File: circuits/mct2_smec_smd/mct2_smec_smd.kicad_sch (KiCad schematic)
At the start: 8 parts

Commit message: 20250306-1
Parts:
- added J?: Conn_02x15_Odd_Even, symbol Connector_Generic:Conn_02x15_Odd_Even
- U? (x7): value ~ -> GW1N-UV2QN48C7/I6; footprint (none) -> Package_DFN_QFN:QFN-48-1EP_6x6mm_P0.4mm_EP4.2x4.2mm_ThermalVias
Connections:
- net GND: now also J?.1 (Pin_1), J?.10 (Pin_10), J?.13 (Pin_13), J?.16 (Pin_16), J?.19 (Pin_19), J?.2 (Pin_2), J?.20 (Pin_20), J?.25 (Pin_25), J?.30 (Pin_30), J?.6 (Pin_6), J?.7 (Pin_7); no longer J?.29 (Pin_29), J?.3 (Pin_3), J?.36 (Pin_36)
- net VDD: no longer J?.4 (Pin_4)
- net DISP_B0: no longer names the net of J?.21 (Pin_21)
- net DISP_B0: no longer U?.28 (IOB5B/SO)
- net DISP_B1: no longer names the net of J?.22 (Pin_22)
- net DISP_B1: no longer U?.29 (IOB5A/SCLK)
- net DISP_B2: no longer names the net of J?.23 (Pin_23)
- net DISP_B2: no longer U?.30 (IOB7B/GCLKC_4)
- net DISP_B3: no longer names the net of J?.24 (Pin_24)
- net DISP_B3: no longer U?.31 (IOB7A/GCLKT_4)
- net DISP_B4: no longer names the net of J?.25 (Pin_25)
- net DISP_B4: no longer U?.32 (IOB13B)
- net DISP_B5: no longer names the net of J?.26 (Pin_26)
- net DISP_B5: no longer U?.33 (IOB13A)
- net DISP_B6: no longer names the net of J?.27 (Pin_27)
- net DISP_B6: no longer U?.34 (IOB18A/SSPI_CS_N)
- net DISP_B7: no longer names the net of J?.28 (Pin_28)
- net DISP_B7: no longer U?.35 (IOB18B/SI)
- net DISP_DE: no longer names the net of J?.34 (Pin_34)
- net DISP_DE: no longer U?.27 (IOL17A)
- net DISP_DISP: no longer names the net of J?.31 (Pin_31)
- net DISP_G0: no longer names the net of U?.44 (IOR3B/D3)
- net DISP_G0: no longer J?.13 (Pin_13)
- net DISP_G1: no longer names the net of U?.45 (IOR3A/D2)
- net DISP_G1: no longer J?.14 (Pin_14)
- net DISP_G2: no longer names the net of U?.46 (IOR1B)
- net DISP_G2: no longer J?.15 (Pin_15)
- net DISP_G3: no longer names the net of U?.47 (IOR1A)
- net DISP_G3: no longer J?.16 (Pin_16)
- net DISP_G4: no longer names the net of U?.38 (IOR13A)
- net DISP_G4: no longer J?.17 (Pin_17)
- net DISP_G5: no longer names the net of U?.39 (IOR13B)
- net DISP_G5: no longer J?.18 (Pin_18)
- net DISP_G6: no longer names the net of U?.40 (IOR11B/GCLKC_2)
- net DISP_G6: no longer J?.19 (Pin_19)
- net DISP_G7: no longer names the net of U?.41 (IOR11A/GCLKT_2)
- net DISP_G7: no longer J?.20 (Pin_20)
- net DISP_HSYNC: no longer names the net of J?.32 (Pin_32)
- net DISP_HSYNC: no longer U?.23 (IOL15A)
- net DISP_PCLK: no longer names the net of J?.30 (Pin_30)
- net DISP_PCLK: no longer U?.22 (IOL15B)
- net DISP_R0: no longer names the net of U?.6 (IOT11A/GCLKT_0)
- net DISP_R0: no longer J?.5 (Pin_5)
- net DISP_R1: no longer names the net of U?.7 (IOT11B/GCLKC_0)
- net DISP_R1: no longer J?.6 (Pin_6)
- net DISP_R2: no longer names the net of U?.8 (IOT9B/TMS)
- net DISP_R2: no longer J?.7 (Pin_7)
- net DISP_R3: no longer names the net of U?.9 (IOT9A/TCK)
- net DISP_R3: no longer J?.8 (Pin_8)
- net DISP_R4: no longer names the net of U?.10 (IOT7B/TDI)
- net DISP_R4: no longer J?.9 (Pin_9)
- net DISP_R5: no longer names the net of U?.11 (IOT7A/TDO)
- net DISP_R5: no longer J?.10 (Pin_10)
- net DISP_R6: no longer names the net of U?.13 (IOT2A/MODE0)
- net DISP_R6: no longer J?.11 (Pin_11)
- net DISP_R7: no longer names the net of U?.48 (IOT16B/RECONFIG_N)
- net DISP_R7: no longer J?.12 (Pin_12)
- net DISP_VSYNC: no longer names the net of J?.33 (Pin_33)
- net DISP_VSYNC: no longer U?.24 (IOL17B)
- new net DISP_ID: J?.14 (Pin_14)
- new net DISP_IO: J?.8 (Pin_8)
- new net DISP_MTP_VPP: J?.23 (Pin_23)
- new net DISP_RST: J?.12 (Pin_12)
- new net DISP_VBAT: J?.27 (Pin_27), J?.29 (Pin_29)
- new net DISP_VCI_EN: J?.4 (Pin_4)
- new net MIPI_CLK_N: J?.3 (Pin_3), U?.22 (IOL15B)
- new net MIPI_CLK_P: J?.5 (Pin_5), U?.23 (IOL15A)
- new net MIPI_D0_N: J?.15 (Pin_15), U?.24 (IOL17B)
- new net MIPI_D0_P: J?.17 (Pin_17), U?.27 (IOL17A)
- new net MIPI_TE: J?.21 (Pin_21)
- new net TP_INT: J?.24 (Pin_24)
- new net TP_RST: J?.22 (Pin_22)
- new net TP_SCL: J?.28 (Pin_28)
- new net TP_SDA: J?.26 (Pin_26)
- new net TP_VCC: J?.18 (Pin_18)
- no-connect marks 5 -> 2
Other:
- note added: "1"
- note added: "2025-02-24 - 2025-03-02"
- note added: "40"
- note added: "BANK0"
- note added: "BANK1"
- note added: "BANK2"
- note added: "BANK3"
- note added: "BANK4"
- note added: "BANK5"
- note added: "Datasheet for TOH323XVT-01C has the pinout inconsistent for: Pin 22 - Drawing: CTP_RST - Module Interface: GND"
- note added: "IOL15A/B and IOL17A/B should support MIPI per LVDS support in UG171 and DS100"
- note added: "Make sure to also refer to the Raydium RM690C0 datasheet for pin definitions"
- note added: "Raydium RM690C0 Datasheet Rev. V0.1 states a maximum DSI bandwidth of 550Mbps per lane. GOWIN DS100 states a maximum MIPI DSI TX rate of 2Gbps per lane. Width x Length x Bit depth x FPS = 262 x 928 x 24 x 60 = 350115840 = 333.90 Mibps/350.12 Mbps"
- note added: "TODO: - Should VPP/MTP be exposed via a separate header for in-circuit programming?"
- note removed: "2025-02-24 - 2025-02-24"
- moved on the sheet: J?, U?A, U?B, U?C, U?D, U?E, U?F, U?G

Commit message: 20250306-2
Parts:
- added J2: Conn_01x07, Connector_PinHeader_2.54mm:PinHeader_1x07_P2.54mm_Vertical, symbol Connector_Generic:Conn_01x07
- added NT1, NT2, NT3, NT4: NetTie_2, symbol Device:NetTie_2
- J1: renamed from J?; value Conn_01x40_Socket -> Input 1x40 FPC; footprint (none) -> Connector_FFC-FPC:TE_4-1734839-0_1x40-1MP_P0.5mm_Horizontal
- J3: renamed from J?; footprint (none) -> Connector_PinHeader_2.54mm:PinHeader_2x10_P2.54mm_Vertical_SMD
- gave numbers to parts that had none: 1
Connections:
- net GND: now also J1.29 (Pin_29), J1.3 (Pin_3), J1.36 (Pin_36), U1.2 (VSS), U1.26 (VSS)
- net JTAG_JTAGSEL_N: now also J2.1 (Pin_1), NT1.2
- net JTAG_MODE0: now also U1.13 (IOT2A/MODE0), J2.6 (Pin_6)
- net JTAG_RECONFIG_N: now also U1.48 (IOT16B/RECONFIG_N), J2.7 (Pin_7)
- net JTAG_TCK: now also J2.3 (Pin_3), NT3.2
- net JTAG_TDI: now also J2.4 (Pin_4), NT4.2
- net JTAG_TDO: now also U1.11 (IOT7A/TDO), J2.5 (Pin_5)
- net JTAG_TMS: now also J2.2 (Pin_2), NT2.2
- net MIPI_TE: now also U1.21 (IOL11B)
- net RGB_B0: now also J1.21 (Pin_21), U1.28 (IOB5B/SO)
- net RGB_B1: now also J1.22 (Pin_22), U1.29 (IOB5A/SCLK)
- net RGB_B2: now also J1.23 (Pin_23), U1.30 (IOB7B/GCLKC_4)
- net RGB_B3: now also J1.24 (Pin_24), U1.31 (IOB7A/GCLKT_4)
- net RGB_B4: now also J1.25 (Pin_25), U1.32 (IOB13B)
- net RGB_B5: now also J1.26 (Pin_26), U1.33 (IOB13A)
- net RGB_B6: now also J1.27 (Pin_27), U1.34 (IOB18A/SSPI_CS_N)
- net RGB_B7: now also J1.28 (Pin_28), U1.35 (IOB18B/SI)
- net RGB_DE: now also J1.34 (Pin_34), U1.17 (IOL5B/LPLL_C_in)
- net RGB_G0: now also J1.13 (Pin_13), U1.3 (IOT16A/JTAGSEL_N), NT1.1
- net RGB_G1: now also J1.14 (Pin_14), U1.4 (IOT14B/GCLKC_1/SDA)
- net RGB_G2: now also J1.15 (Pin_15), U1.5 (IOT14A/GCLKT_1/SCL)
- net RGB_G3: now also J1.16 (Pin_16), U1.6 (IOT11A/GCLKT_0)
- net RGB_G4: now also J1.17 (Pin_17), U1.7 (IOT11B/GCLKC_0)
- net RGB_G5: now also J1.18 (Pin_18), U1.8 (IOT9B/TMS), NT2.1
- net RGB_G6: now also J1.19 (Pin_19), U1.9 (IOT9A/TCK), NT3.1
- net RGB_G7: now also J1.20 (Pin_20), U1.10 (IOT7B/TDI), NT4.1
- net RGB_HSYNC: now also J1.32 (Pin_32), U1.15 (IOL4A/LPLL_T_fb)
- net RGB_PCLK: now also J1.30 (Pin_30), U1.14 (IOL4B/LPLL_C_fb)
- net RGB_R0: now also J1.5 (Pin_5), U1.38 (IOR13A)
- net RGB_R1: now also J1.6 (Pin_6), U1.39 (IOR13B)
- net RGB_R2: now also J1.7 (Pin_7), U1.40 (IOR11B/GCLKC_2)
- net RGB_R3: now also J1.8 (Pin_8), U1.41 (IOR11A/GCLKT_2)
- net RGB_R4: now also J1.9 (Pin_9), U1.42 (IOR5B/MO/D6)
- net RGB_R5: now also J1.10 (Pin_10), U1.43 (IOR5A/MI/D7)
- net RGB_R6: now also J1.11 (Pin_11), U1.44 (IOR3B/D3)
- net RGB_R7: now also J1.12 (Pin_12), U1.45 (IOR3A/D2)
- net RGB_VSYNC: now also J1.33 (Pin_33), U1.16 (IOL5A/LPLL_T_in)
- net VDD: now also J1.4 (Pin_4)
- net RGB_EN: now reaches U1.18 (IOL6A/GCLKT_7)
- net RGB_EN: now also J1.31 (Pin_31)
- net DISP_IO renamed DISP_IOVCC
- net DISP_MTP_VPP: no longer names the net of J3.23 (Pin_23)
- no-connect marks 2 -> 8
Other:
- note added: "2025-02-24 - 2025-03-06"
- note added: "TODO: replace pin header with proper footprint for OK-23GF030-04"
- note removed: "2025-02-24 - 2025-03-02"
- note removed: "Datasheet for TOH323XVT-01C has the pinout inconsistent for: Pin 22 - Drawing: CTP_RST - Module Interface: GND"
- note removed: "TODO: - Should VPP/MTP be exposed via a separate header for in-circuit programming?"
- note removed: "TODO: find out if these pins have important alternate functions and move data pins if they do"
- moved on the sheet: J1, U1A, U1C, U1D, U1E, U1F, U1G

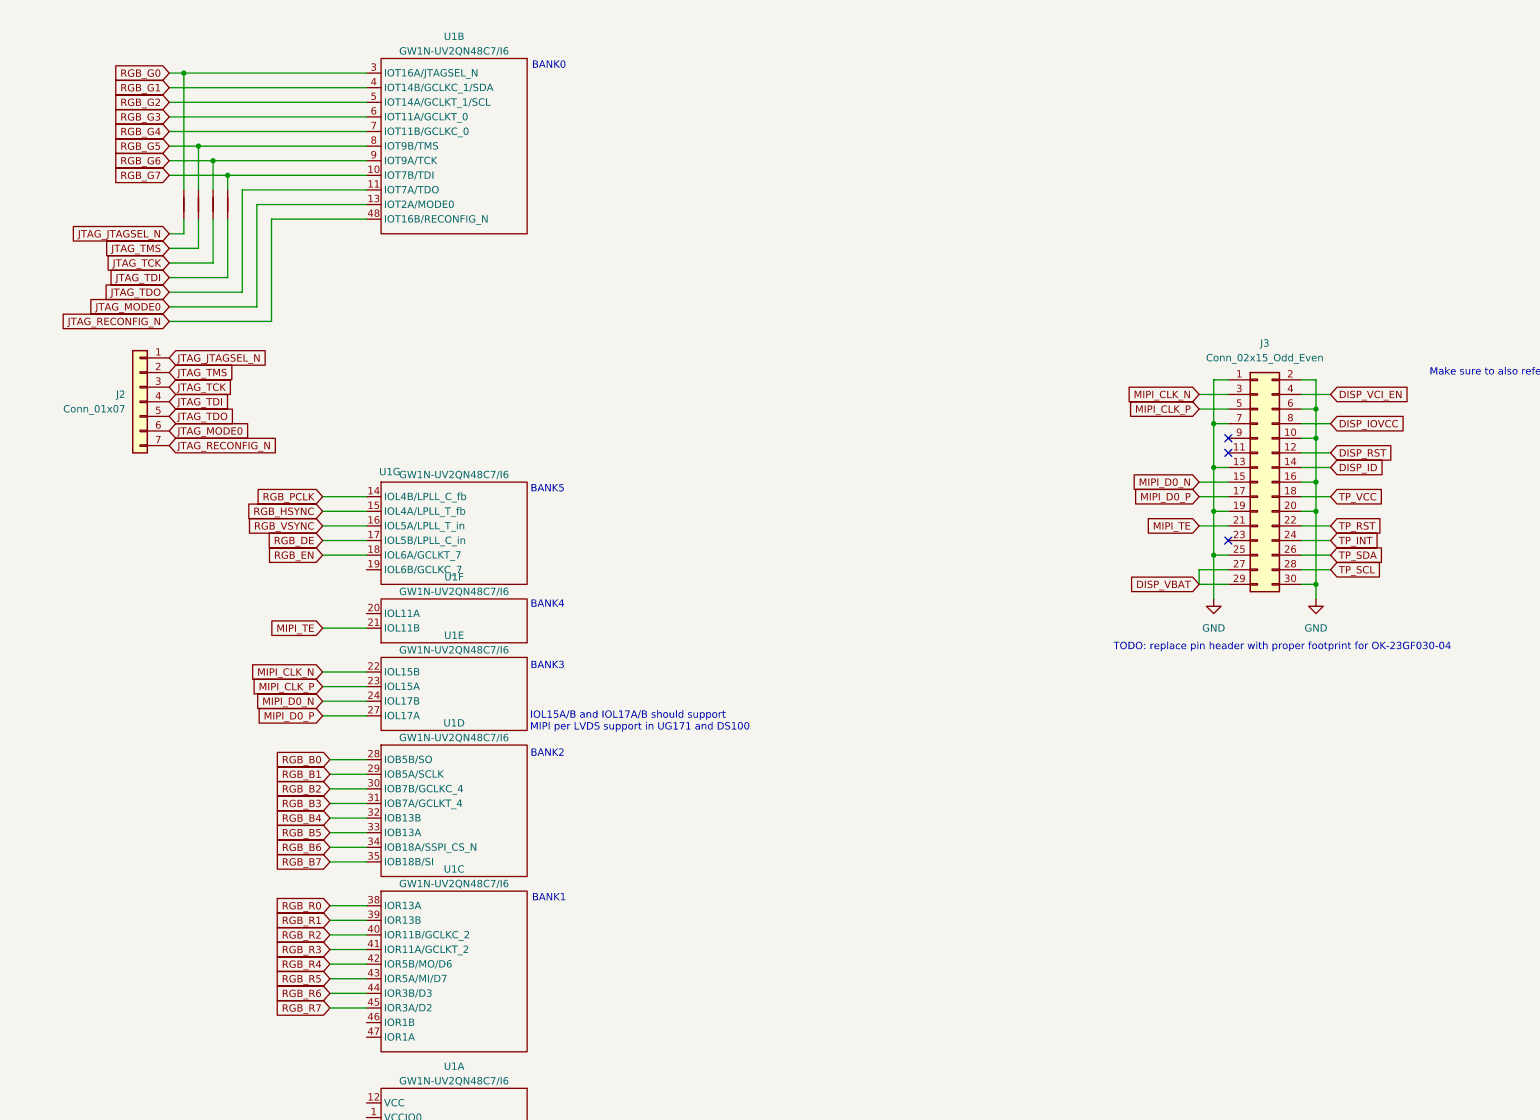
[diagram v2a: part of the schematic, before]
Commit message: 20250311-1
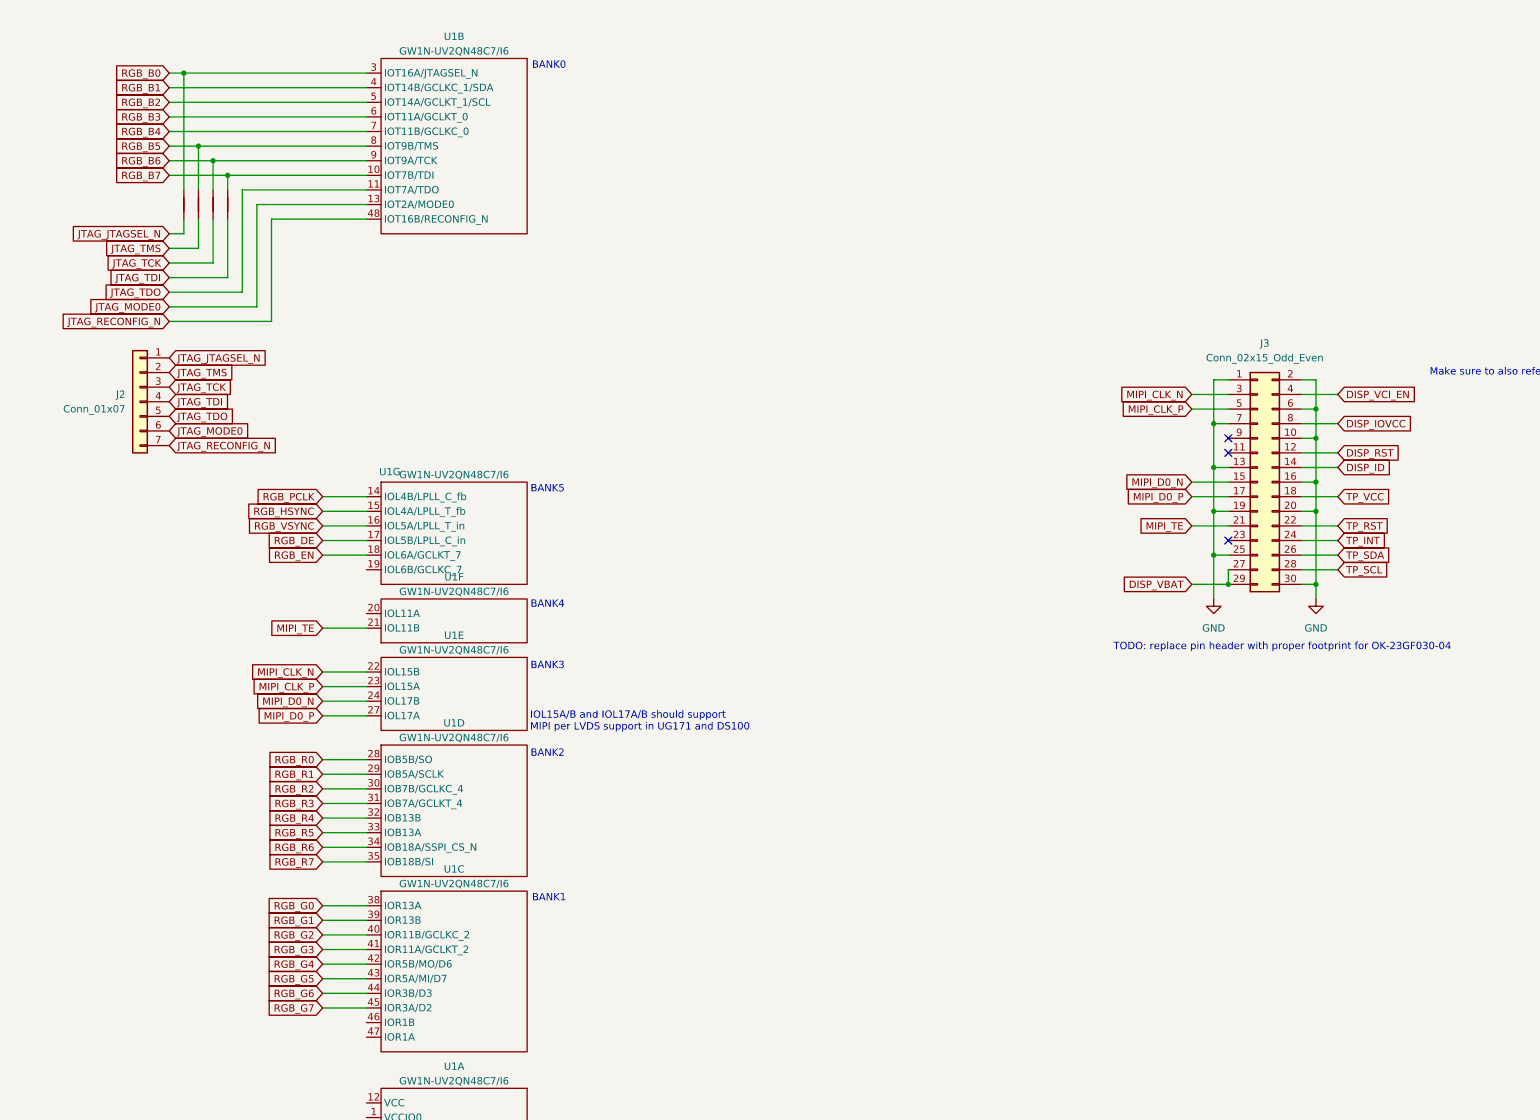
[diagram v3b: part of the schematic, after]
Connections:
- net RGB_B0: now also NT1.1, U1.3 (IOT16A/JTAGSEL_N); no longer U1.28 (IOB5B/SO)
- net RGB_B1: now also U1.4 (IOT14B/GCLKC_1/SDA); no longer U1.29 (IOB5A/SCLK)
- net RGB_B2: now also U1.5 (IOT14A/GCLKT_1/SCL); no longer U1.30 (IOB7B/GCLKC_4)
- net RGB_B3: now also U1.6 (IOT11A/GCLKT_0); no longer U1.31 (IOB7A/GCLKT_4)
- net RGB_B4: now also U1.7 (IOT11B/GCLKC_0); no longer U1.32 (IOB13B)
- net RGB_B5: now also NT2.1, U1.8 (IOT9B/TMS); no longer U1.33 (IOB13A)
- net RGB_B6: now also NT3.1, U1.9 (IOT9A/TCK); no longer U1.34 (IOB18A/SSPI_CS_N)
- net RGB_B7: now also NT4.1, U1.10 (IOT7B/TDI); no longer U1.35 (IOB18B/SI)
- net RGB_G0: now also U1.38 (IOR13A); no longer NT1.1, U1.3 (IOT16A/JTAGSEL_N)
- net RGB_G1: now also U1.39 (IOR13B); no longer U1.4 (IOT14B/GCLKC_1/SDA)
- net RGB_G2: now also U1.40 (IOR11B/GCLKC_2); no longer U1.5 (IOT14A/GCLKT_1/SCL)
- net RGB_G3: now also U1.41 (IOR11A/GCLKT_2); no longer U1.6 (IOT11A/GCLKT_0)
- net RGB_G4: now also U1.42 (IOR5B/MO/D6); no longer U1.7 (IOT11B/GCLKC_0)
- net RGB_G5: now also U1.43 (IOR5A/MI/D7); no longer NT2.1, U1.8 (IOT9B/TMS)
- net RGB_G6: now also U1.44 (IOR3B/D3); no longer NT3.1, U1.9 (IOT9A/TCK)
- net RGB_G7: now also U1.45 (IOR3A/D2); no longer NT4.1, U1.10 (IOT7B/TDI)
- net RGB_R0: now also U1.28 (IOB5B/SO); no longer U1.38 (IOR13A)
- net RGB_R1: now also U1.29 (IOB5A/SCLK); no longer U1.39 (IOR13B)
- net RGB_R2: now also U1.30 (IOB7B/GCLKC_4); no longer U1.40 (IOR11B/GCLKC_2)
- net RGB_R3: now also U1.31 (IOB7A/GCLKT_4); no longer U1.41 (IOR11A/GCLKT_2)
- net RGB_R4: now also U1.32 (IOB13B); no longer U1.42 (IOR5B/MO/D6)
- net RGB_R5: now also U1.33 (IOB13A); no longer U1.43 (IOR5A/MI/D7)
- net RGB_R6: now also U1.34 (IOB18A/SSPI_CS_N); no longer U1.44 (IOR3B/D3)
- net RGB_R7: now also U1.35 (IOB18B/SI); no longer U1.45 (IOR3A/D2)

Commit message: 20250313-1
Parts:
- added U2: ~, Package_TO_SOT_SMD:SOT-23-8, symbol mediacow:TCA9416
- J2: footprint Connector_PinHeader_2.54mm:PinHeader_1x07_P2.54mm_Vertical -> Connector_PinHeader_2.54mm:PinHeader_1x07_P2.54mm_Vertical_SMD_Pin1Left
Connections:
- net GND: now also U2. (VCCB)
- net MIPI_CLK_N: now also U1.23 (IOL15A); no longer U1.22 (IOL15B)
- net MIPI_CLK_P: now also U1.22 (IOL15B); no longer U1.23 (IOL15A)
- net MIPI_D0_N: now also U1.21 (IOL11B); no longer U1.24 (IOL17B)
- net MIPI_D0_P: now also U1.20 (IOL11A); no longer U1.27 (IOL17A)
- net MIPI_TE: now also U1.24 (IOL17B); no longer U1.21 (IOL11B)
- net RGB_DE: now also U1.18 (IOL6A/GCLKT_7); no longer U1.17 (IOL5B/LPLL_C_in)
- net RGB_EN: now also U1.15 (IOL4A/LPLL_T_fb); no longer U1.18 (IOL6A/GCLKT_7)
- net RGB_HSYNC: now also U1.16 (IOL5A/LPLL_T_in); no longer U1.15 (IOL4A/LPLL_T_fb)
- net RGB_VSYNC: now also U1.17 (IOL5B/LPLL_C_in); no longer U1.16 (IOL5A/LPLL_T_in)
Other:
- note added: "2025-02-24 - 2025-03-13"
- note removed: "2025-02-24 - 2025-03-06"
- moved on the sheet: J2, U1A, U1C, U1D, U1E, U1F, U1G
